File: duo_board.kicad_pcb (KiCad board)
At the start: 4 copper layers, 167 x 122.9 mm, 55 parts, among them J1 TRRS, J2 2171790001, J3 Conn_01x04_Pin, U1 STM32F103C8Tx, U3 AMS1117-3.3

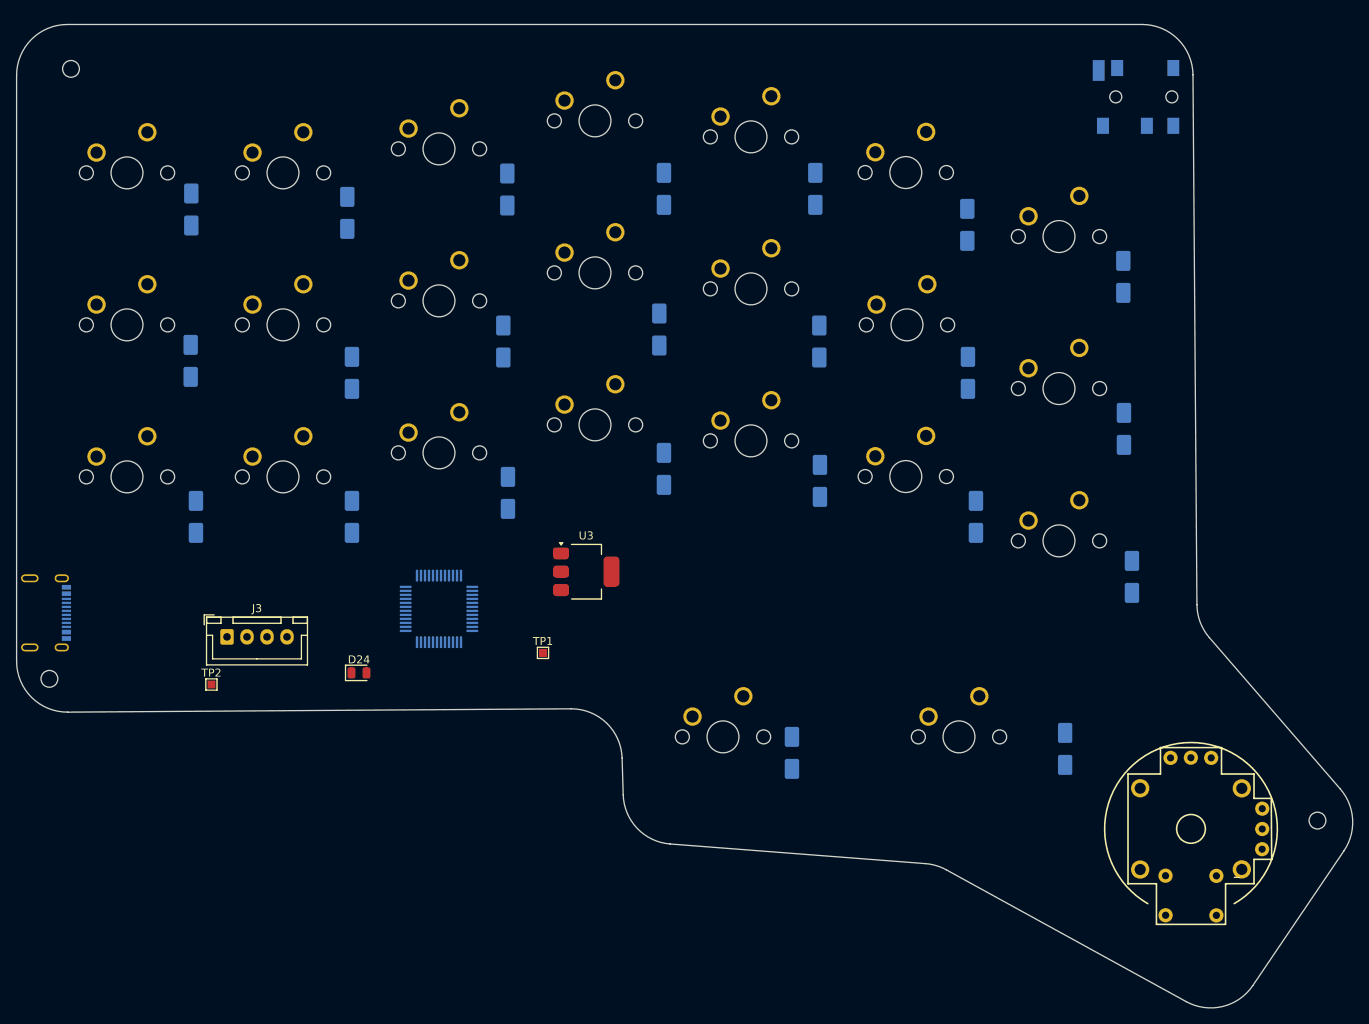
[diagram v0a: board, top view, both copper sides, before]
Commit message: routed, ready for production?
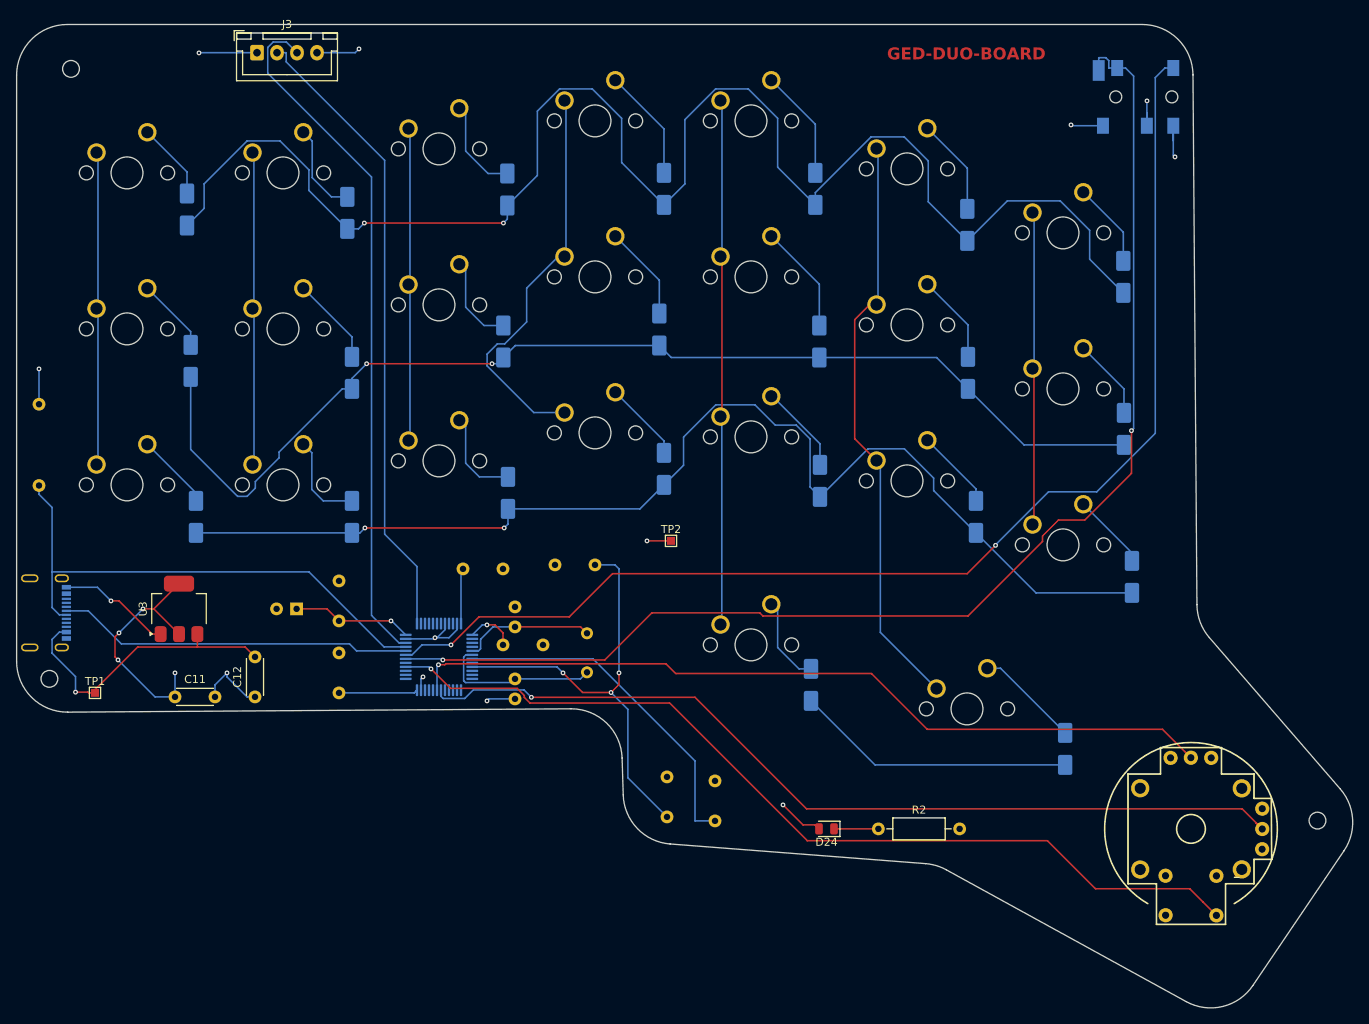
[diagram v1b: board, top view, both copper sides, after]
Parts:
- added C1: 100nF, Capacitor_THT:C_Disc_D4.3mm_W1.9mm_P5.00mm, B.Cu at (102.5, 113.5)
- added C10: 22pF, Capacitor_THT:C_Disc_D3.0mm_W1.6mm_P2.50mm, B.Cu at (124.5, 111.8)
- added C11: 22uF, Capacitor_THT:C_Disc_D4.3mm_W1.9mm_P5.00mm, F.Cu at (82.0, 114.0)
- added C12: 22uF, Capacitor_THT:C_Disc_D4.3mm_W1.9mm_P5.00mm, F.Cu at (92.0, 114.0)
- added C2: 100nF, Capacitor_THT:C_Disc_D4.3mm_W1.9mm_P5.00mm, B.Cu at (123.0, 107.5)
- added C3: 100nF, Capacitor_THT:C_Disc_D4.3mm_W1.9mm_P5.00mm, B.Cu at (102.5, 104.5)
- added C4: 100nF, Capacitor_THT:C_Disc_D4.3mm_W1.9mm_P5.00mm, B.Cu at (118.0, 98.0)
- added C5: 10uF, Capacitor_THT:CP_Radial_Tantal_D5.5mm_P2.50mm, B.Cu at (97.2, 103.0)
- added C6: 10nF, Capacitor_THT:C_Disc_D4.3mm_W1.9mm_P5.00mm, B.Cu at (134.5, 97.5)
- added C7: 1uF, Capacitor_THT:C_Disc_D4.3mm_W1.9mm_P5.00mm, B.Cu at (143.5, 129.0)
- added C8: 100nF, Capacitor_THT:C_Disc_D4.3mm_W1.9mm_P5.00mm, B.Cu at (149.5, 129.5)
- added C9: 22pF, Capacitor_THT:C_Disc_D3.0mm_W1.6mm_P2.50mm, B.Cu at (124.5, 102.8)
- added R1: 1K5, Resistor_THT:R_Axial_DIN0207_L6.3mm_D2.5mm_P10.16mm_Horizontal, B.Cu at (65.0, 77.4)
- added R2: 1K5, Resistor_THT:R_Axial_DIN0207_L6.3mm_D2.5mm_P10.16mm_Horizontal, F.Cu at (169.9, 130.5)
- added Y1: 16Mhz, Crystal:Crystal_HC49-4H_Vertical, B.Cu at (133.5, 106.0)
- moved MX12 81.9 mm to (154.0, 61.5)
- moved MX7 78.7 mm to (193.0, 56.0)
- moved J3 73.1 mm to (92.2, 33.5)
- moved MX8 64.0 mm to (76.0, 68.0)
- moved D24 61.6 mm to (163.4, 130.5), turned to 180 degrees
- moved TP2 60.2 mm to (144.0, 94.5)
- moved MX11 59.7 mm to (134.5, 61.5)
- moved MX9 58.7 mm to (95.5, 68.0)
- moved MX10 58.6 mm to (115.0, 65.0)
- moved TP1 56.2 mm to (72.0, 113.5)
- moved U3 51.1 mm to (82.5, 103.0), turned to 90 degrees
- moved MX4 46.6 mm to (134.5, 42.0)
- moved MX19 45.9 mm to (154.0, 81.5)
- moved MX5 45.0 mm to (154.0, 42.0)
- moved MX3 44.8 mm to (115.0, 45.5)
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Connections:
- J1 pad 2: unconnected-(J1-Pad2) -> USART1_RX
- J1 pad 3: unconnected-(J1-Pad3) -> USART1_TX
- J1 pad 4: unconnected-(J1-Pad4) -> USART1_TX
- J1 pad 5: unconnected-(J1-Pad5) -> GND
- J1 pad 6: unconnected-(J1-Pad6) -> +3.3V
- J1 pad 7: unconnected-(J1-Pad7) -> +3.3V
- U1 pad 18: unconnected-(U1-PB0-Pad18) -> /X_AXIS
- U1 pad 19: unconnected-(U1-PB1-Pad19) -> /Y_AXIS
- U1 pad 28: unconnected-(U1-PB15-Pad28) -> /BTN_PIN
- U1 pad 30: unconnected-(U1-PA9-Pad30) -> USART1_TX
- U1 pad 31: unconnected-(U1-PA10-Pad31) -> USART1_RX
- U2 pad B1A: unconnected-(U2-SEL+-PadB1A) -> /BTN_PIN
- U2 pad B2A: unconnected-(U2-SEL--PadB2A) -> GND
- U2 pad H1: unconnected-(U2-H+-PadH1) -> GND
- U2 pad H2: unconnected-(U2-H-PadH2) -> /Y_AXIS
- U2 pad H3: unconnected-(U2-H--PadH3) -> +3.3V
- U2 pad S1: Net-(U2-SHIELD-PadS1) -> GND
- U2 pad S2: Net-(U2-SHIELD-PadS1) -> GND
- U2 pad S3: Net-(U2-SHIELD-PadS1) -> GND
- U2 pad S4: Net-(U2-SHIELD-PadS1) -> GND
- U2 pad V1: unconnected-(U2-V+-PadV1) -> +3.3V
- U2 pad V2: unconnected-(U2-V-PadV2) -> /X_AXIS
- U2 pad V3: unconnected-(U2-V--PadV3) -> GND
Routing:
- net ROW0: track 0.00 -> 193.5 mm, vias 0 -> 2
- net USART1_TX: track 0.00 -> 158.8 mm, vias 0 -> 2
- net USART1_RX: track 0.00 -> 152.4 mm, vias 0 -> 2
- net +3.3V: track 0.00 -> 152.1 mm, vias 0 -> 15
- net ROW2: track 0.00 -> 146.0 mm, vias 0 -> 2
- net ROW1: track 0.00 -> 142.8 mm, vias 0 -> 2
- net /BTN_PIN: track 0.00 -> 114.3 mm, vias 0 -> 1
- net /X_AXIS: track 0.00 -> 112.3 mm, vias 0 -> 1
- net /Y_AXIS: track 0.00 -> 102.2 mm, vias 0 -> 1
- net /SWDIO: track 0.00 -> 86.5 mm
- net /SWCLK: track 0.00 -> 79.3 mm
- net COL5: track 0.00 -> 73.5 mm
- net /USB_D+: track 0.00 -> 66.2 mm
- net COL4: track 0.00 -> 65.9 mm
- net GND: track 0.00 -> 53.3 mm, vias 0 -> 7
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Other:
- board text added: "GED-DUO-BOARD"
